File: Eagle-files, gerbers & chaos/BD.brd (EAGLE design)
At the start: 100 x 81.3 mm, 57 parts, among them IC1 TL072P, Q1 BC546A, Q2 BC556A, Q3 BC546A, Q4 BC546A, Q5 BC546A, Q6 BC546A, X1 ACC+TRIG, X2 OUT, X3 SUPPLY

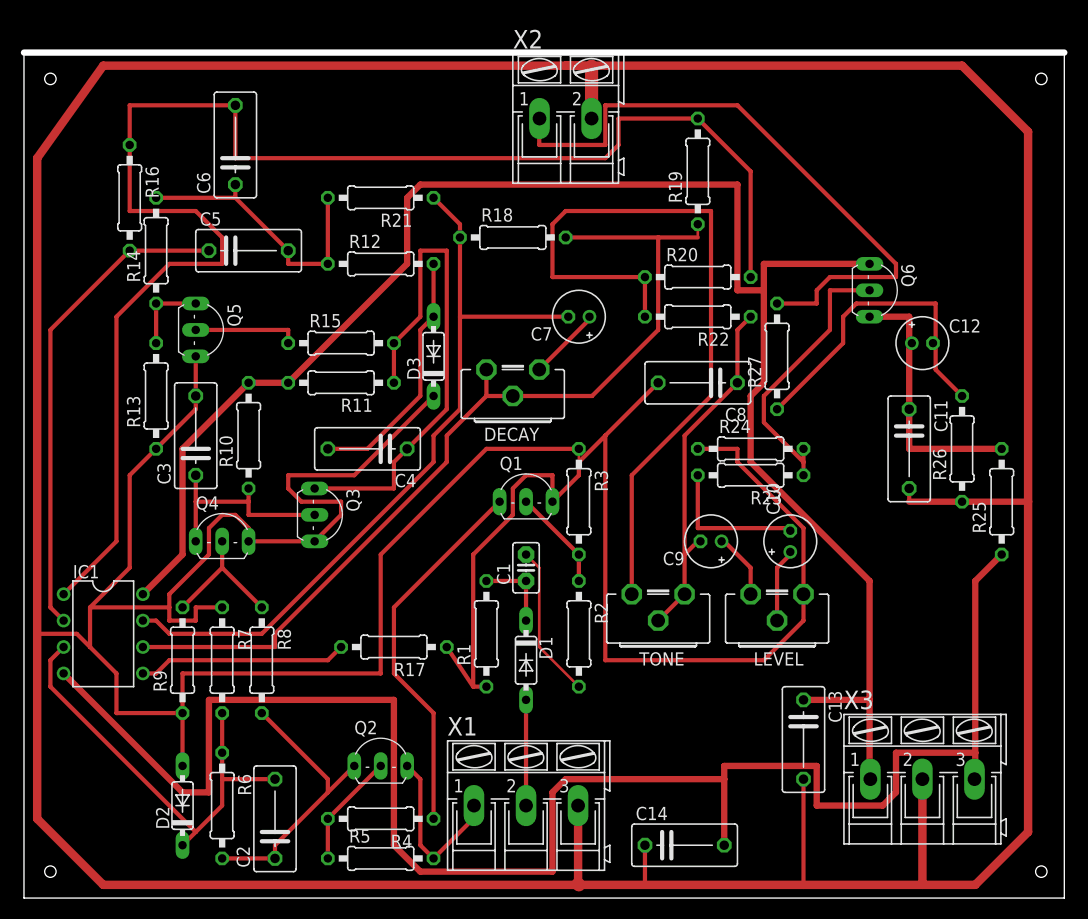
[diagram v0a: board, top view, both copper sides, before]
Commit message: Cleaned up, added PDF of schematics
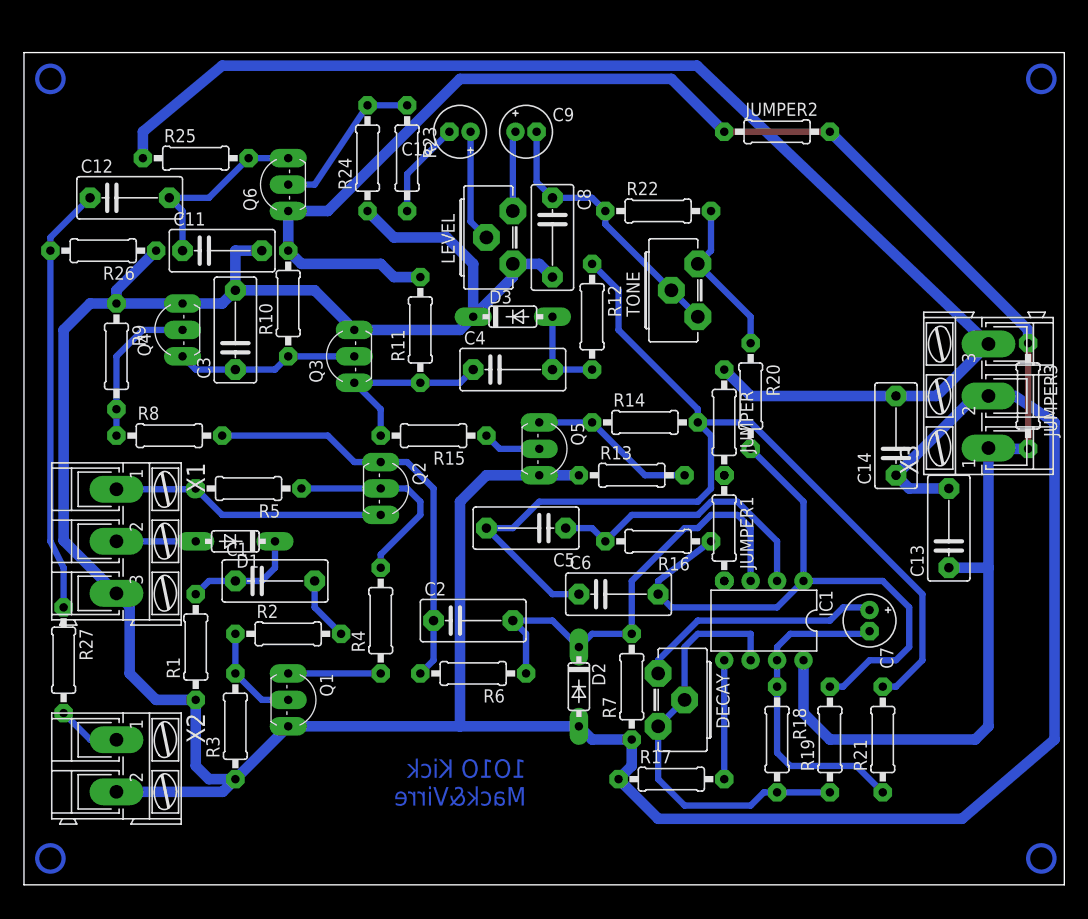
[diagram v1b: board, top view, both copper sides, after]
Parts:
- added JUMPER, JUMPER1, JUMPER2, JUMPER3: 0, resistor:0207/10
- C1: value 0.1 -> 0,1u; device capacitor-wima:C2.5-2 -> rcl:C075-042X103
- C12: device rcl:E2-5 -> rcl:C075-042X103
- moved R26 84.7 mm to (7.62, 61.0), turned to 180 degrees
- moved R25 84.2 mm to (16.5, 69.8), turned to 0 degrees
- moved C12 77.5 mm to (10.2, 66.0)
- moved X2 75.7 mm to (8.89, 11.4), turned to 270 degrees
- moved R27 74.5 mm to (3.81, 21.6), turned to 270 degrees
- moved R21 71.0 mm to (82.5, 14.0), turned to 90 degrees
- moved C11 68.7 mm to (19.1, 61.0), turned to 0 degrees
- moved IC1 63.5 mm to (71.1, 25.4), turned to 180 degrees
- moved R16 60.6 mm to (61.0, 33.0), turned to 180 degrees
- moved Q6 59.3 mm to (24.1, 67.3), turned to 90 degrees
- moved C6 56.8 mm to (57.1, 27.9), turned to 0 degrees
- moved R19 56.1 mm to (77.5, 14.0)
- moved R18 54.5 mm to (72.4, 14.0), turned to 270 degrees
- moved C10 50.6 mm to (41.9, 72.4), turned to 180 degrees
- moved R14 49.8 mm to (59.7, 44.5), turned to 0 degrees
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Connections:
- new net N$18: JUMPER.2, JUMPER1.1
- new net N$23: IC1.4, JUMPER1.2
- net +15V: now also JUMPER2.1, JUMPER2.2, JUMPER3.1, JUMPER3.2
- net -15V: now also JUMPER.1; no longer IC1.4
- net N$30: now also C12.2; no longer C12.+
- net N$31: now also C12.1; no longer C12.-
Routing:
- net GND: track 680.6 -> 330.8 mm
- net N$20: track 143.8 -> 62.2 mm
- net N$33: track 27.5 -> 100.7 mm
- net N$24: track 73.5 -> 15.3 mm
- net N$32: track 61.5 -> 6.14 mm
- net N$5: track 89.8 -> 41.3 mm
- net N$21: track 73.2 -> 31.4 mm
- net -15V: track 162.9 -> 125.4 mm
- net N$14: track 48.9 -> 18.1 mm
- net N$6: track 36.3 -> 8.89 mm
- net N$19: track 46.9 -> 27.8 mm
- net N$22: track 7.44 -> 23.8 mm
- net N$12: track 24.2 -> 8.89 mm
- net N$9: track 27.4 -> 40.7 mm
- net N$28: track 27.1 -> 15.5 mm
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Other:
- board size 100 x 81.3 mm -> 100 x 80 mm
- board text added: "1O1O Kick Mack&Virre"
